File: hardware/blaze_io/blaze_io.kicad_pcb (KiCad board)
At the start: 4 copper layers, 70 x 70 mm, 58 parts, among them J1 Conn_01x30_Pin, J2 Conn_01x30_Socket, J3 Conn_01x04, J4 Conn_01x04, J5 Conn_01x03_Pin, J6 Conn_01x03_Pin, J7 Conn_01x03_Pin, J8 Conn_01x03_Pin, J9 JTAG, Q1 AO4892, Q2 AO4892, SW1 SW_SPST, SW2 SW_SPDT, U1 TCAN1044VDDFR, U2 4081, U3 STM32H503KBUx

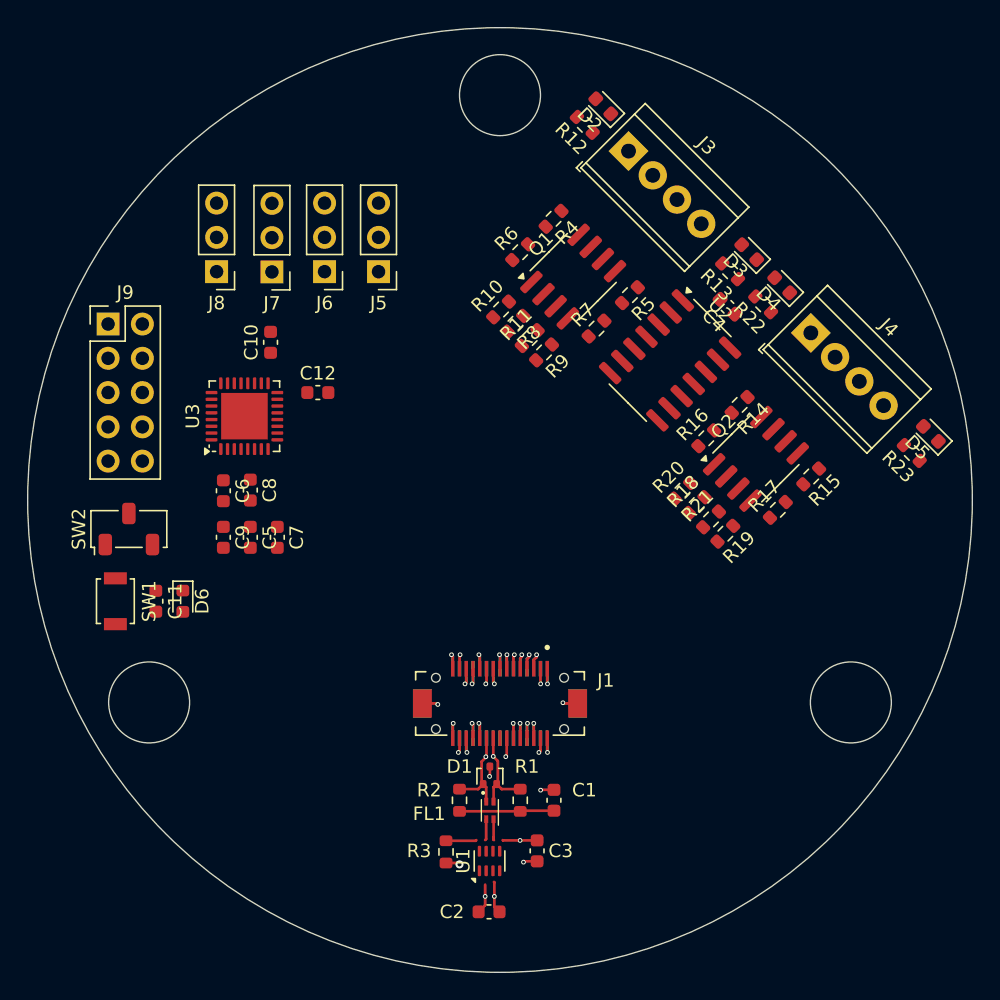
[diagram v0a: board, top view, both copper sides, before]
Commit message: PCB Work
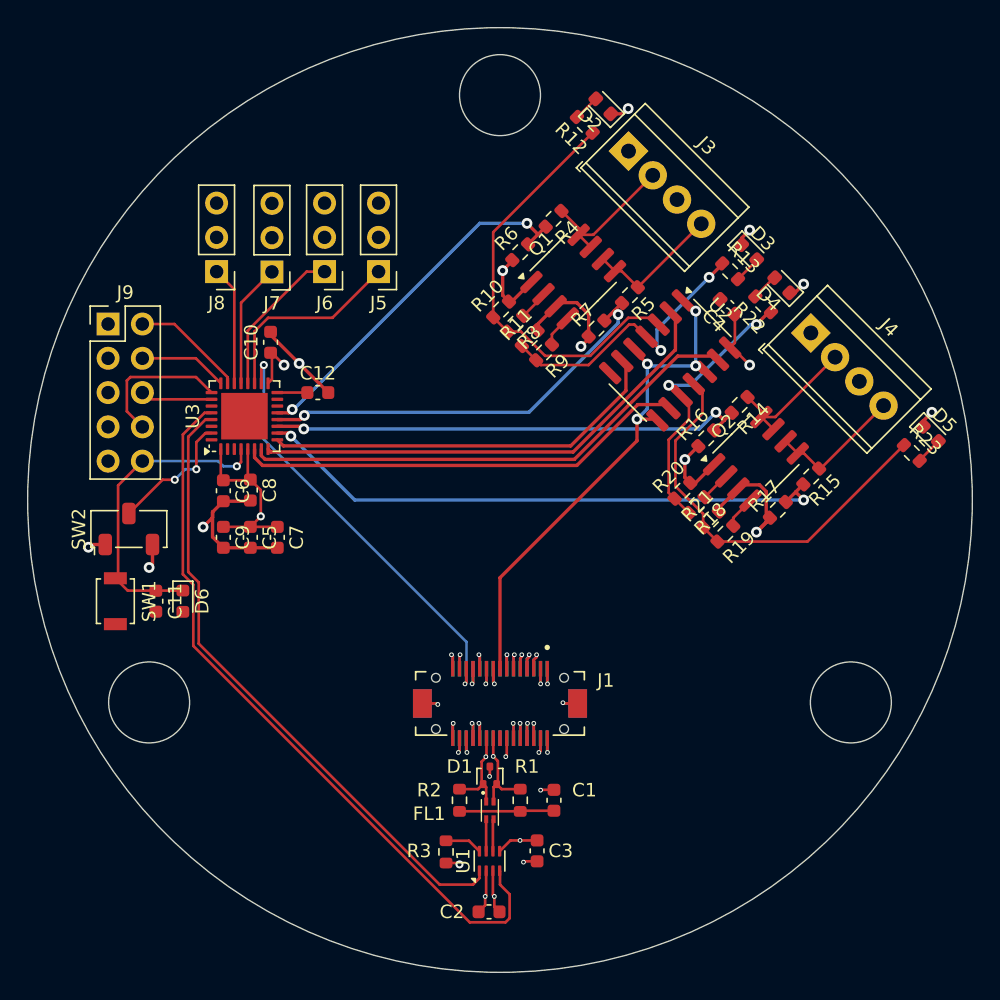
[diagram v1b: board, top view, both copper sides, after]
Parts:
- turned D3 to -45 degrees
- turned D5 to -45 degrees
- turned R13 to -45 degrees
- turned R18 to -135 degrees
- turned R23 to -45 degrees
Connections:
- J1 pad 25: Net-(J1-Pin_25) -> +5V
- J1 pad 26: Net-(J1-Pin_26) -> +5V
- J2 pad 5: Net-(J1-Pin_26) -> +5V
- J2 pad 6: Net-(J1-Pin_25) -> +5V
- J3 pad 1: GND -> VBATT
- J3 pad 3: GND -> VBATT
- J4 pad 1: GND -> VBATT
- J4 pad 3: GND -> VBATT
- R10 pad 1: /FET_A -> Net-(R10-Pad1)
- R12 pad 1: /FET_A -> Net-(R10-Pad1)
- R18 pad 2: /FET_C -> Net-(R18-Pad2)
- R20 pad 1: /FET_C -> Net-(R18-Pad2)
- R22 pad 1: /FET_C -> Net-(R18-Pad2)
- R8 pad 2: /FET_A -> Net-(R10-Pad1)
- U2 pad 10: /FET_C -> Net-(R18-Pad2)
- U2 pad 3: /FET_A -> Net-(R10-Pad1)
- U3 pad 10: /FET_A_SENSE -> /FET_D_SENSE
- U3 pad 11: /FET_B_SENSE -> /FET_C_SENSE
- U3 pad 12: /FET_C_SENSE -> /FET_B_SENSE
- U3 pad 13: /FET_D_SENSE -> /FET_A_SENSE
- U3 pad 6: /FET_A -> /FET_C
- U3 pad 7: /FET_B -> /FET_D
- U3 pad 8: /FET_C -> /FET_A
- U3 pad 9: /FET_D -> /FET_B
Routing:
- net VBATT: track 4.53 -> 65.4 mm
- net GND: track 18.2 -> 73.1 mm, vias 10 -> 21
- net /CANRX: track 0.00 -> 54.6 mm
- net +5V: track 33.1 -> 84.8 mm, vias 7 -> 6
- net /CANTX: track 0.00 -> 46.8 mm
- net /FET_D_SENSE: track 0.00 -> 43.7 mm, vias 0 -> 2
- net /ARM: track 2.10 -> 40.1 mm, vias 1 -> 4
- net /FET_D: track 0.00 -> 37.7 mm
- net /FET_A: track 0.00 -> 36.3 mm
- net /FET_C_SENSE: track 0.00 -> 35.8 mm, vias 0 -> 2
- net /FET_C: track 0.00 -> 33.6 mm
- net /FET_B_SENSE: track 0.00 -> 31.6 mm, vias 0 -> 2
- net Net-(R10-Pad1): track 0.00 -> 31.6 mm
- net Net-(R19-Pad2): track 0.00 -> 30.8 mm
- net /PPS: track 2.33 -> 32.5 mm, vias 1 -> 2
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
